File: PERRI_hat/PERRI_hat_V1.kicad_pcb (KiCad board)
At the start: 2 copper layers, 65 x 90 mm, 62 parts, among them J1 ST5-80-1.00-L-D-P-TR, J2 ST5-80-1.00-L-D-P-TR, Q1 MMST3904-7-F

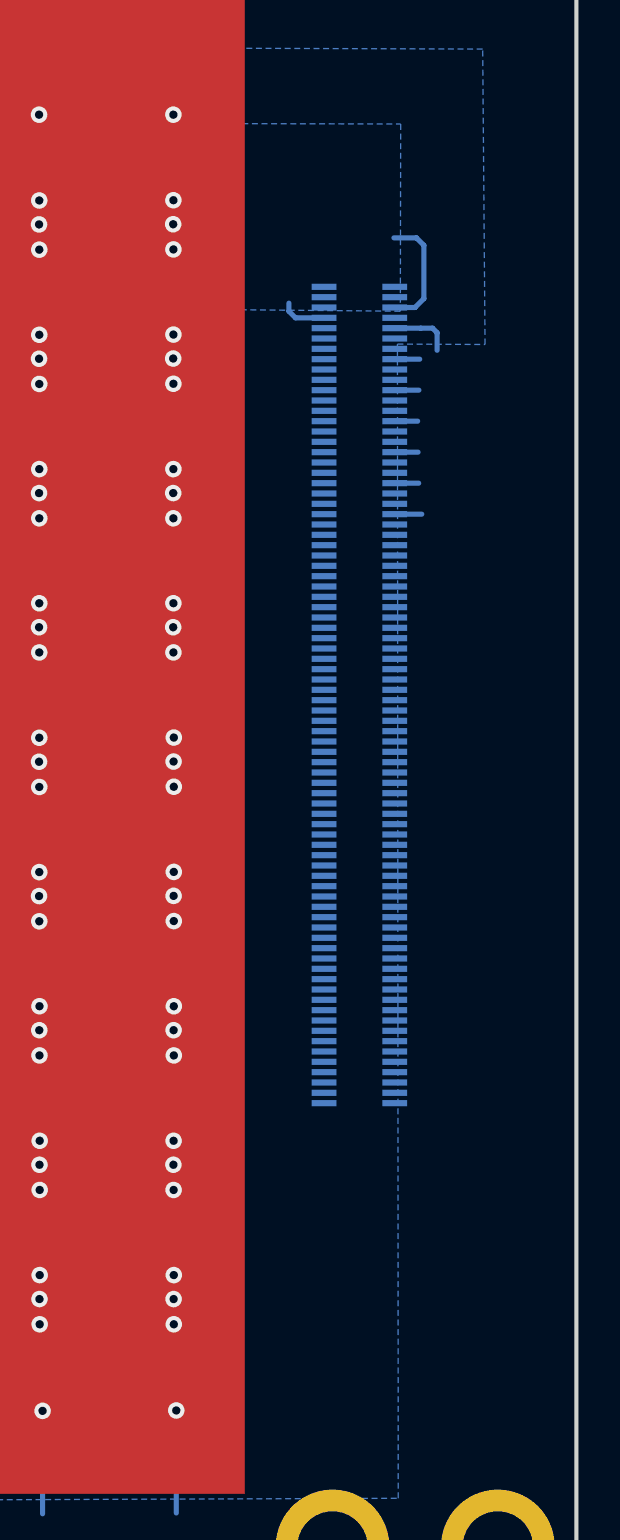
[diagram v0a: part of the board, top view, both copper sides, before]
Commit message: Add files via upload
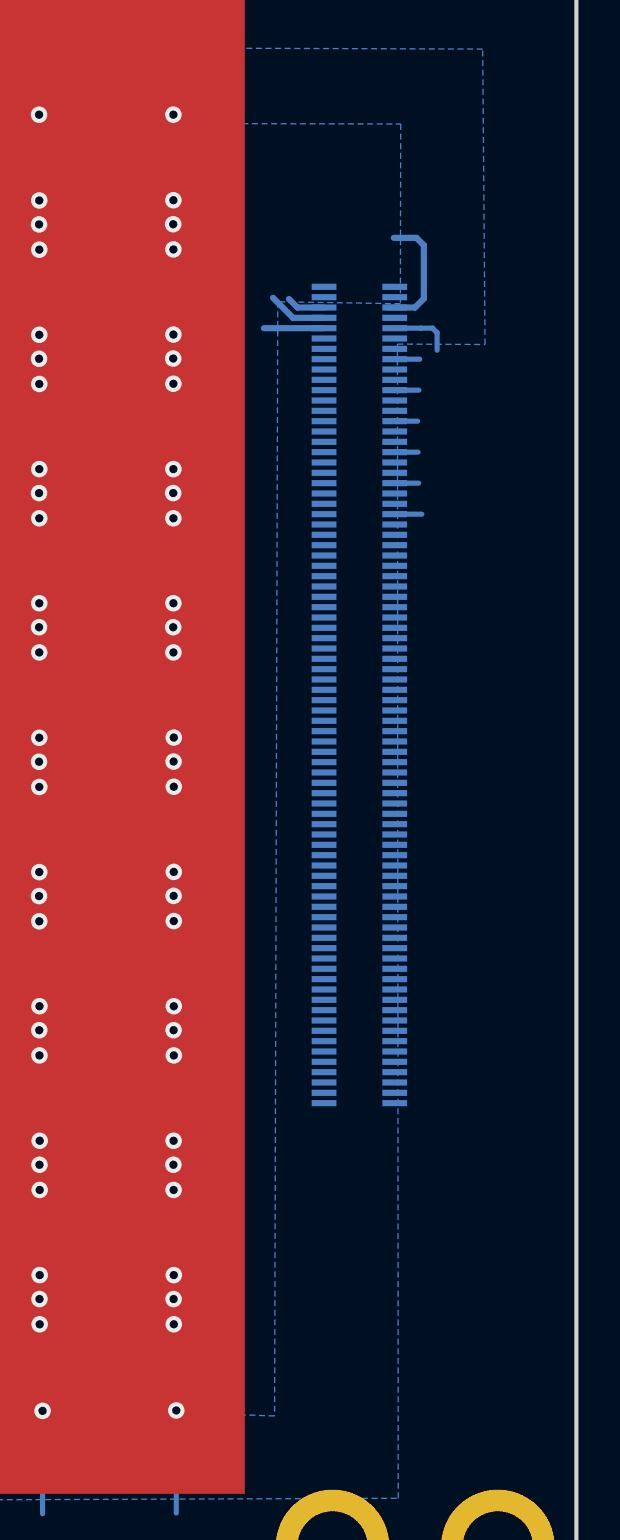
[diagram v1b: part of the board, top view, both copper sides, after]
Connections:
- J2 pad 09: unconnected-(J2-Pad09) -> /12V_FROM_SURF
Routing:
- net /12V_FROM_SURF: track 7.99 -> 13.8 mm
